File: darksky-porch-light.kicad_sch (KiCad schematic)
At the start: 15 parts, among them J1 Motion, J2 FTDI, Q1 QM6006D, U1 ESP32-WROOM-32E, U2 AD8606ARZ

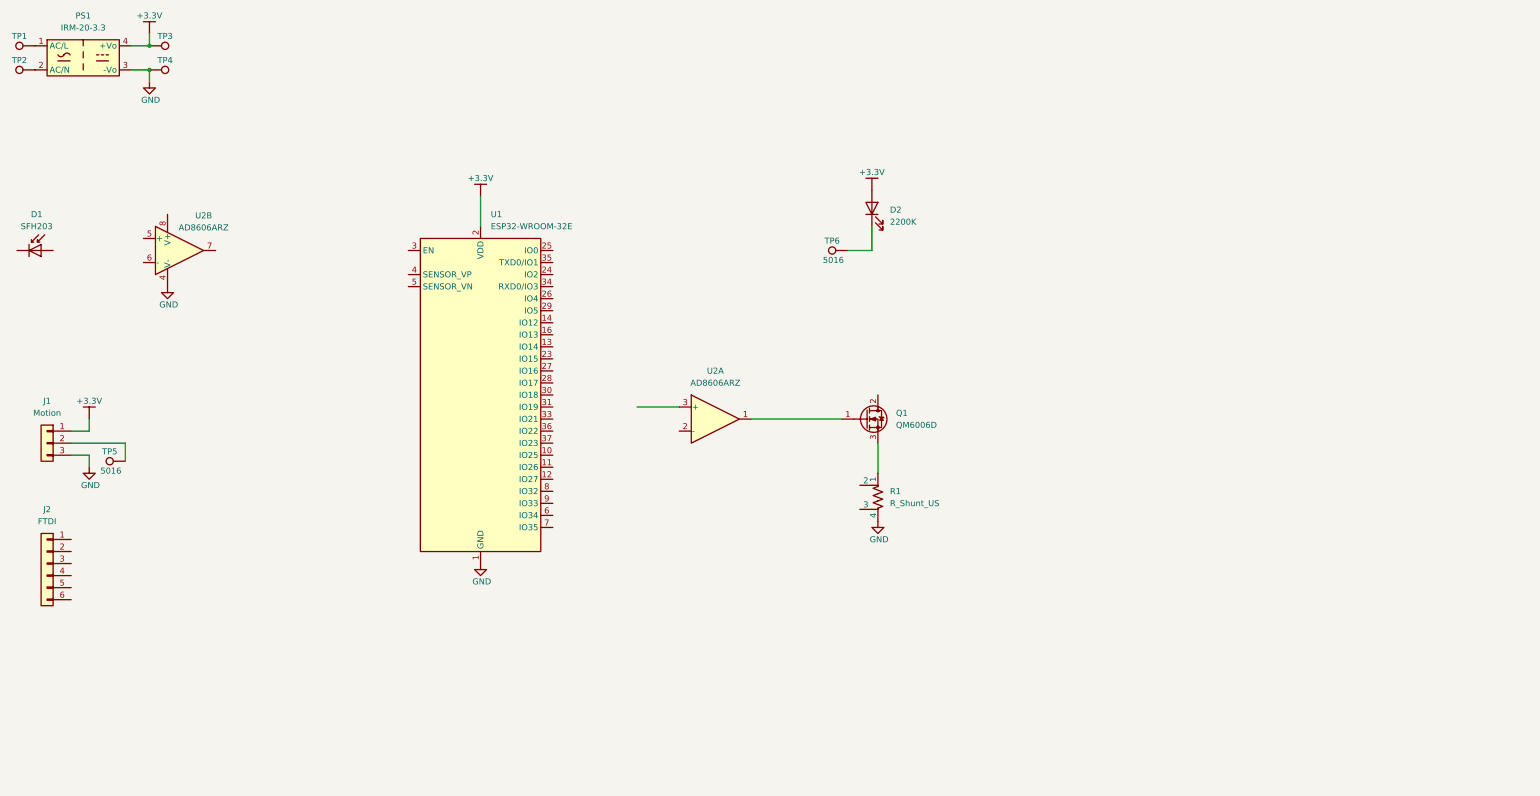
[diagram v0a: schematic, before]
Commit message: layout
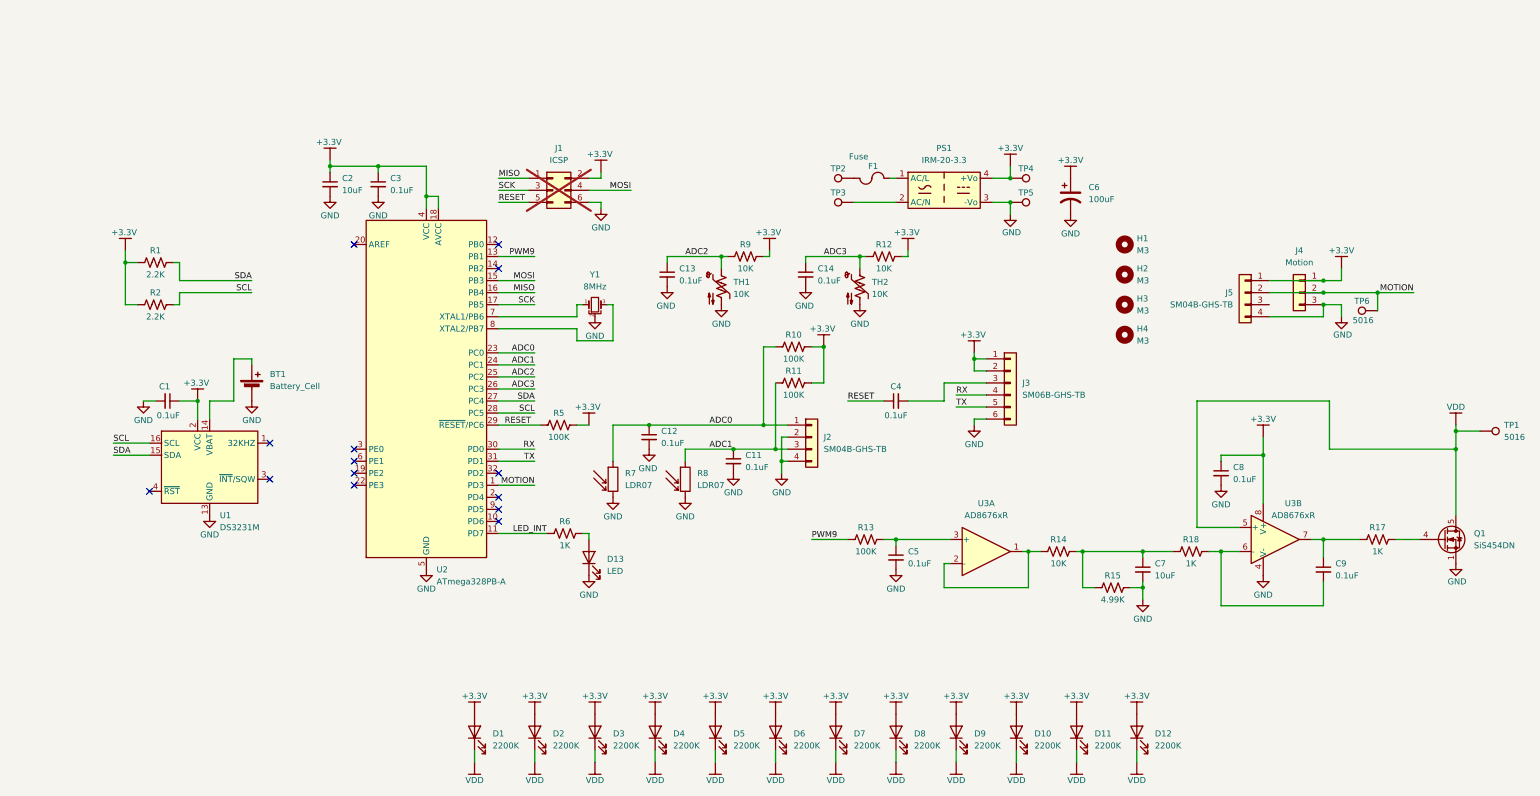
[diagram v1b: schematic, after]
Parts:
- removed D1: SFH203, LED_THT:LED_D5.0mm_IRGrey, symbol Sensor_Optical:SFH203
- removed J2: FTDI, Connector_PinHeader_2.54mm:PinHeader_1x06_P2.54mm_Vertical, symbol Connector_Generic:Conn_01x06
- removed Q1: QM6006D, Package_TO_SOT_SMD:TO-252-2, symbol Transistor_FET:QM6006D
- removed R1: R_Shunt_US, Resistor_SMD:R_Shunt_Vishay_WSK2512_6332Metric_T1.19mm, symbol Device:R_Shunt_US
- removed TP6: 5016, jannett_footprints:TestPoint_Keystone_5016_Compact, symbol Connector:TestPoint
- removed U1: ESP32-WROOM-32E, RF_Module:ESP32-WROOM-32D, symbol RF_Module:ESP32-WROOM-32E
- removed U2: AD8606ARZ, Package_SO:SOIC-8_3.9x4.9mm_P1.27mm, symbol Amplifier_Operational:AD8606ARZ
- added BT1: Battery_Cell, Battery:BatteryHolder_Keystone_3002_1x2032, symbol Device:Battery_Cell
- added C1, C11, C12, C13, C14, C3, C4, C5, C8, C9: 0.1uF, Capacitor_SMD:C_0603_1608Metric, symbol Device:C_Small
- added C2, C7: 10uF, Capacitor_SMD:C_0603_1608Metric, symbol Device:C_Small
- added C6: 100uF, Capacitor_SMD:CP_Elec_6.3x5.4_Nichicon, symbol Device:C_Polarized_US
- added D10, D11, D12, D2, D3, D4, D5, D6, D7, D8, D9: 2200K, LED_SMD:LED_PLCC_2835_Handsoldering, symbol Device:LED
- added D13: LED, LED_SMD:LED_0603_1608Metric_Pad1.05x0.95mm_HandSolder, symbol Device:LED
- added F1: Fuse, Fuse:Fuseholder_Littelfuse_Nano2_154x, symbol jannett_symbols:Fuse
- added H1, H2, H3, H4: M3, MountingHole:MountingHole_3.2mm_M3, symbol Mechanical:MountingHole
- added J1: ICSP, Connector_PinSocket_2.00mm:PinSocket_2x03_P2.00mm_Vertical, symbol Connector_Generic:Conn_02x03_Odd_Even
- added J2, J5: SM04B-GHS-TB, Connector_JST:JST_GH_SM04B-GHS-TB_1x04-1MP_P1.25mm_Horizontal, symbol Connector_Generic:Conn_01x04
- added J3: SM06B-GHS-TB, Connector_JST:JST_GH_SM06B-GHS-TB_1x06-1MP_P1.25mm_Horizontal, symbol Connector_Generic:Conn_01x06
- added Q1: SiS454DN, Package_SO:Vishay_PowerPAK_1212-8_Single, symbol Transistor_FET:SiS454DN
- added R1, R2: 2.2K, Resistor_SMD:R_0603_1608Metric, symbol Device:R_US
- added R10, R11, R13, R5: 100K, Resistor_SMD:R_0603_1608Metric, symbol Device:R_US
- added R12, R14, R9: 10K, Resistor_SMD:R_0603_1608Metric, symbol Device:R_US
- added R15: 4.99K, Resistor_SMD:R_0603_1608Metric, symbol Device:R_US
- added R17, R18, R6: 1K, Resistor_SMD:R_0603_1608Metric, symbol Device:R_US
- added R7, R8: LDR07, OptoDevice:R_LDR_5.1x4.3mm_P3.4mm_Vertical, symbol Sensor_Optical:LDR07
- added TH1, TH2: 10K, Resistor_SMD:R_0603_1608Metric, symbol Device:Thermistor_NTC_US
- added TP1: 5016, jannett_footprints:TestPoint_Keystone_5016_Vias, symbol Connector:TestPoint
- added U1: DS3231M, Package_SO:SOIC-16W_7.5x10.3mm_P1.27mm, symbol Timer_RTC:DS3231M
- added U2: ATmega328PB-A, Package_QFP:TQFP-32_7x7mm_P0.8mm, symbol MCU_Microchip_ATmega:ATmega328PB-A
- added U3: AD8676xR, Package_SO:SOIC-8_3.9x4.9mm_P1.27mm, symbol Amplifier_Operational:AD8676xR
- added Y1: 8MHz, Crystal:Resonator_SMD_Murata_CSTxExxV-3Pin_3.0x1.1mm_HandSoldering, symbol Device:Crystal_GND2_Small
- renumbered D2 to D1, J1 to J4, TP1 to TP2, TP2 to TP3, TP3 to TP4, TP4 to TP5, TP5 to TP6
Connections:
- net +3.3V: now also C1.1, C2.1, C3.1, C6.1, C8.1, D10.2 (A), D11.2 (A), D12.2 (A), D2.2 (A), D3.2 (A), D4.2 (A), D5.2 (A), D6.2 (A), D7.2 (A), D8.2 (A), D9.2 (A), J1.2 (Pin_2), J3.1 (Pin_1), J3.2 (Pin_2), J5.1 (Pin_1), R1.1, R10.2, R11.2, R12.2, R2.1, R5.2, R9.2, U1.2 (VCC), U2.18 (AVCC), U2.4 (VCC), U3.8 (V+)
- net GND: now also BT1.2 (-), C1.2, C11.2, C12.2, C13.2, C14.2, C2.2, C3.2, C5.2, C6.2, C7.2, C8.2, D13.1 (K), J1.6 (Pin_6), J2.2 (Pin_2), J2.4 (Pin_4), J3.6 (Pin_6), J5.4 (Pin_4), Q1.1 (S), Q1.2 (S), Q1.3 (S), R15.2, R7.2, R8.2, TH1.2, TH2.2, U1.10 (GND), U1.11 (GND), U1.12 (GND), U1.13 (GND), U1.5 (GND), U1.6 (GND), U1.7 (GND), U1.8 (GND), U1.9 (GND), U2.21 (GND), U2.5 (GND), U3.4 (V-), Y1.2
- net VDD: now reaches D1.1 (K)
- net VDD: now also D10.1 (K), D11.1 (K), D12.1 (K), D2.1 (K), D3.1 (K), D4.1 (K), D5.1 (K), D6.1 (K), D7.1 (K), D8.1 (K), D9.1 (K), Q1.5 (D), TP1.1, U3.5 (+)
- net MOTION: now reaches J4.2 (Pin_2), TP6.1
- net MOTION: now also J5.2 (Pin_2), U2.1 (PD3)
- net at PS1.1 (AC/L): now also F1.2; no longer TP2.1
- new net: Q1.4 (G), R17.2
- new net: U2.7 (XTAL1/PB6), Y1.1
- new net: U2.8 (XTAL2/PB7), Y1.3
- new net: BT1.1 (+), U1.14 (VBAT)
- new net: R14.1, U3.1, U3.2 (-)
- new net: C7.1, R14.2, R15.1, R18.1
- new net: C9.2, R18.2, U3.6 (-)
- new net: C9.1, R17.1, U3.7
- new net: C5.1, R13.2, U3.3 (+)
- new net: C4.2, J3.3 (Pin_3)
- new net: D13.2 (A), R6.2
- new net: F1.1, TP2.1
- new net ADC0: C12.1, J2.1 (Pin_1), R10.1, R7.1, U2.23 (PC0)
- new net ADC1: C11.1, J2.3 (Pin_3), R11.1, R8.1, U2.24 (PC1)
- new net ADC2: C13.1, R9.1, TH1.1, U2.25 (PC2)
- new net ADC3: C14.1, R12.1, TH2.1, U2.26 (PC3)
- new net LED_INT: R6.1, U2.11 (PD7)
- new net MISO: J1.1 (Pin_1), U2.16 (PB4)
- new net MOSI: J1.4 (Pin_4), U2.15 (PB3)
- new net PWM9: R13.1, U2.13 (PB1)
- new net RESET: C4.1, J1.5 (Pin_5), R5.1, U2.29 (~{RESET}/PC6)
- new net RX: J3.4 (Pin_4), U2.30 (PD0)
- new net SCK: J1.3 (Pin_3), U2.17 (PB5)
- new net SCL: R2.2, U1.16 (SCL), U2.28 (PC5)
- new net SDA: R1.2, U1.15 (SDA), U2.27 (PC4)
- new net TX: J3.5 (Pin_5), U2.31 (PD1)
- no-connect marks 0 -> 14
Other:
- moved on the sheet: D1, J4, PS1, TP2, TP3, TP4, TP5, TP6
